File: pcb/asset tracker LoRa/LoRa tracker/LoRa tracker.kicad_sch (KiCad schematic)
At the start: 4 parts

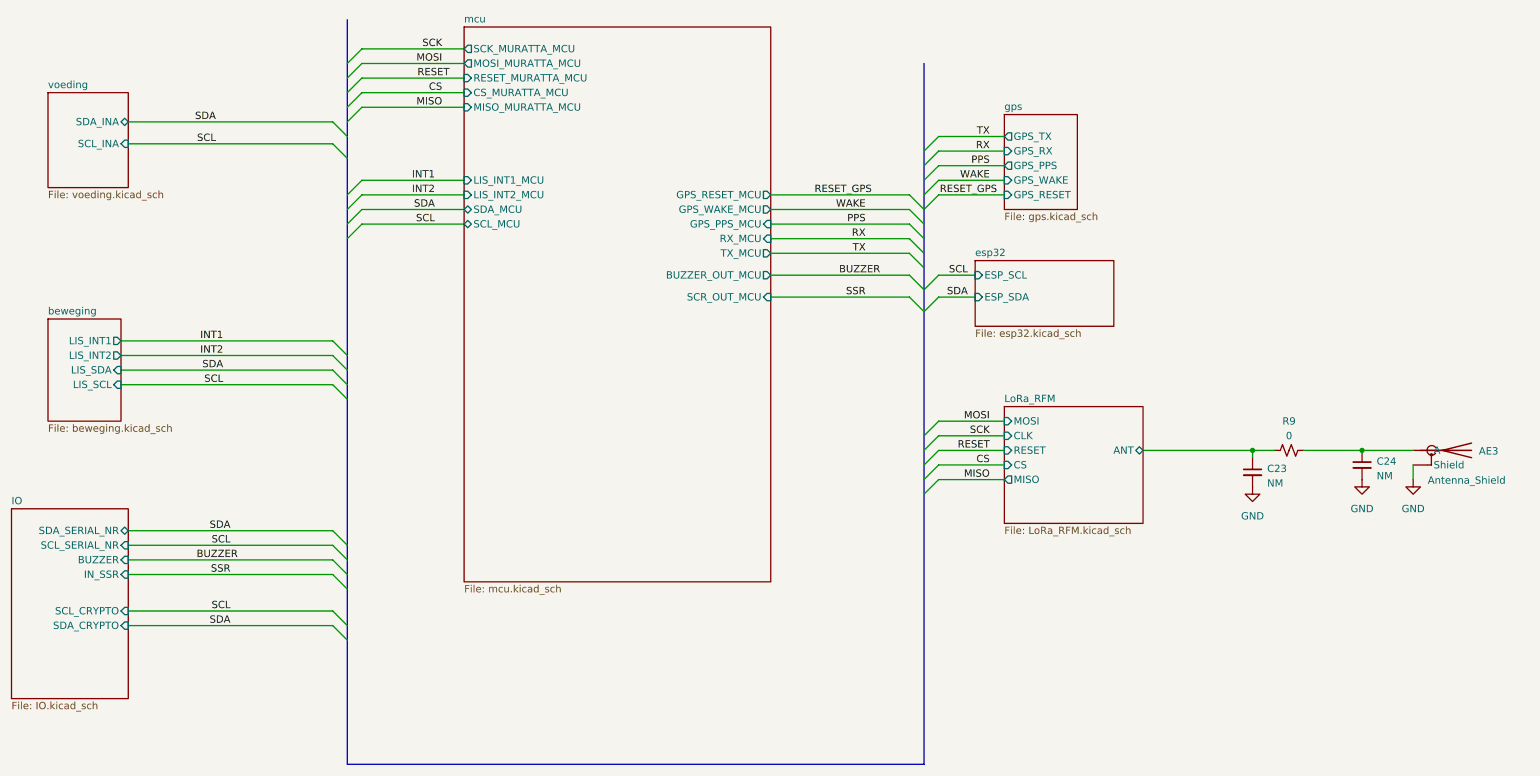
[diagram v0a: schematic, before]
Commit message: fgnhb
fgdh
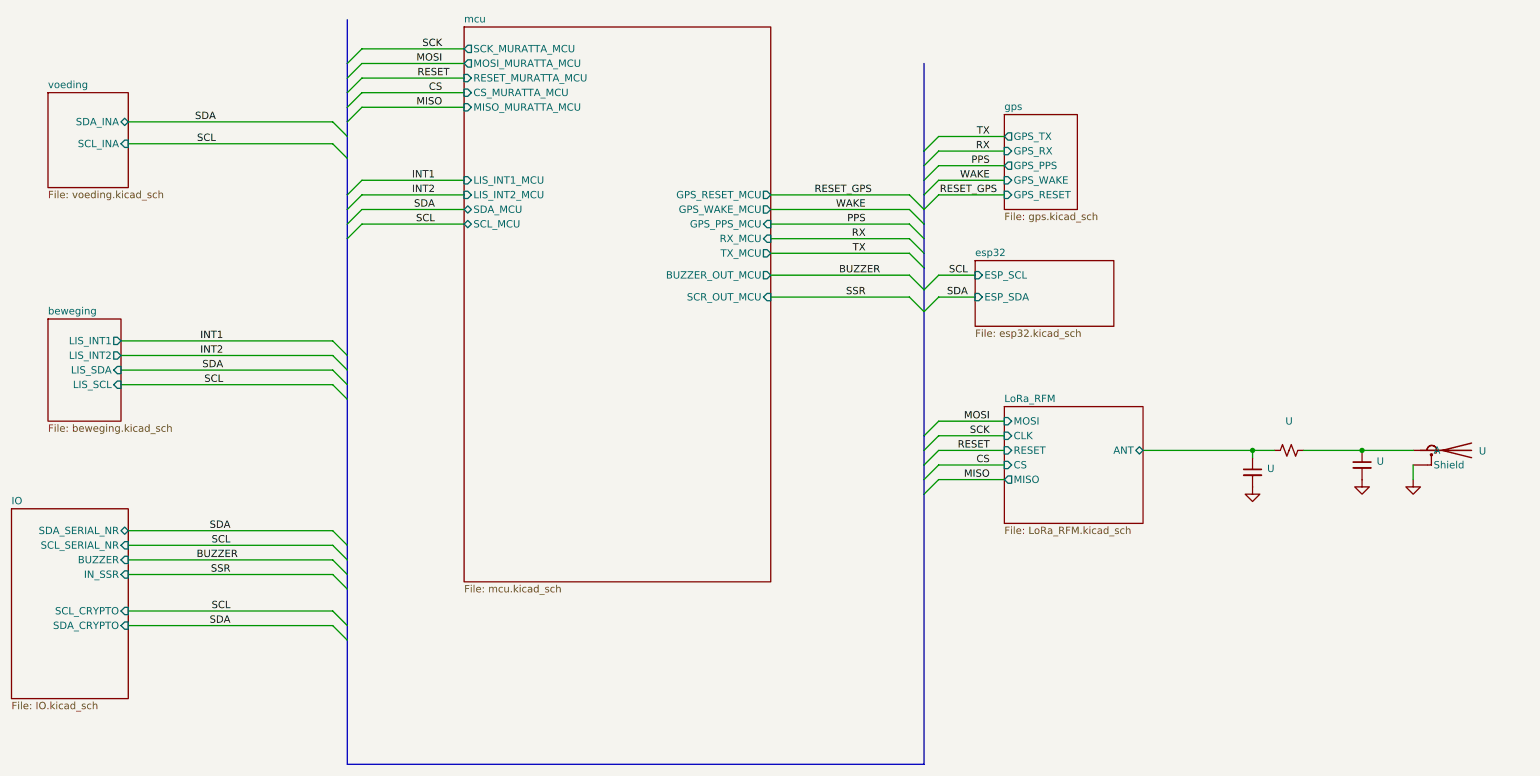
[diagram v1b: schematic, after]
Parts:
- U: renamed from R9; value 0 -> (none); footprint vanalles:0603RL -> (none)
- U: renamed from C23; value NM -> (none); footprint vanalles:0603 -> (none)
- U: renamed from AE3; value Antenna_Shield -> (none); footprint connectors_user:ufl connector -> (none)
- U: renamed from C24; value NM -> (none); footprint vanalles:0603 -> (none)
